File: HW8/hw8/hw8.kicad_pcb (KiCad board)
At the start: 2 copper layers, 27 parts, among them J1 Barrel_Jack, J2 Conn_01x02_Pin, J3 Comm 1 Terminal, J4 Conn_01x02_Pin, J5 Comm 2 Terminal, K1 SANYOU_SRD_Form_C, K2 SANYOU_SRD_Form_C, Q1 BC337, Q2 BC337, U1 LM317_TO-220, U2 PC817, U3 PC817

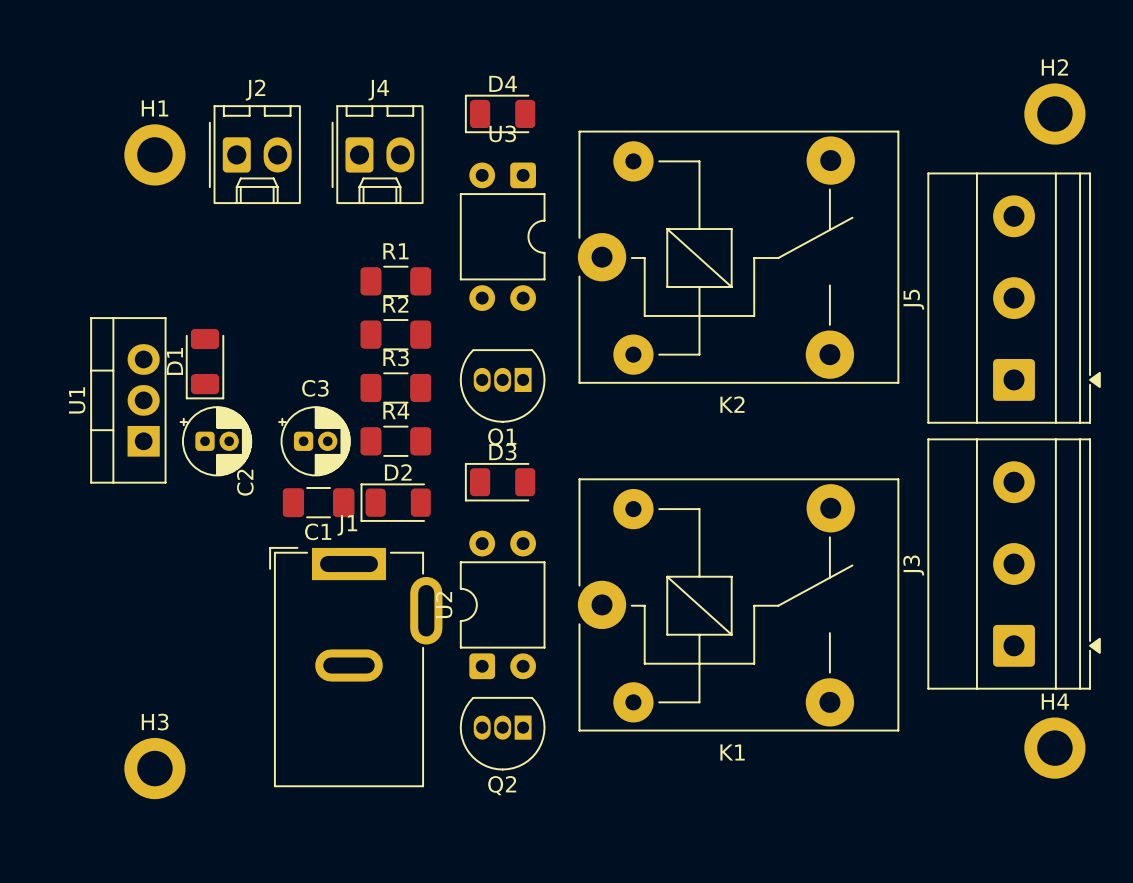
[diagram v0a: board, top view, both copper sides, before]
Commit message: hw9 done
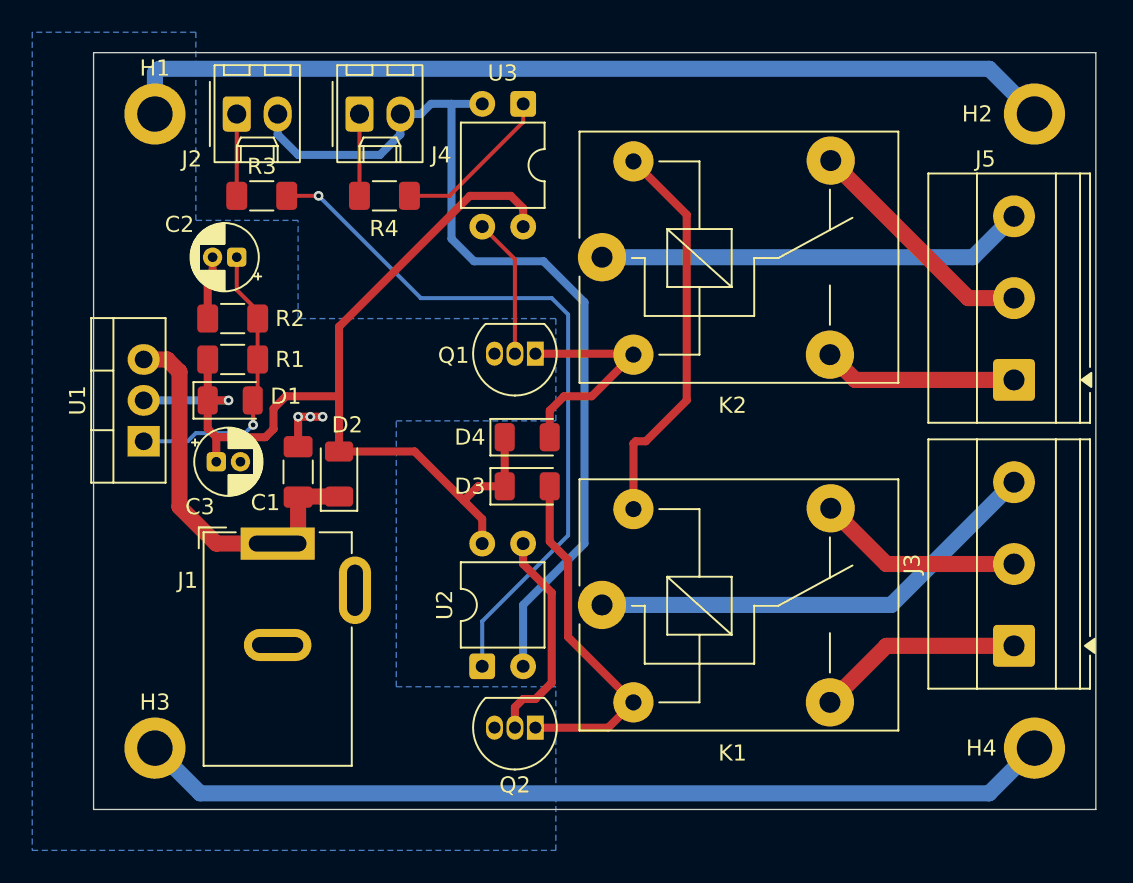
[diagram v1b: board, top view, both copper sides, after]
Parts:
- moved D4 20.1 mm to (119.6, 49.3)
- moved R4 15.3 mm to (110.8, 34.3)
- moved R3 14.6 mm to (103.2, 34.3)
- moved C2 11.6 mm to (101.6, 38.1), turned to 180 degrees
- moved R1 11.2 mm to (101.3, 44.5)
- moved R2 10.2 mm to (101.3, 41.9)
- moved C3 5.57 mm to (100.3, 50.8)
- moved J1 4.61 mm to (104.1, 55.9)
- moved U3 4.44 mm to (119.4, 28.6)
- moved D2 4.09 mm to (108.0, 51.6), turned to 90 degrees
- moved D1 2.87 mm to (101.2, 47.0), turned to 0 degrees
- moved H1 2.54 mm to (96.5, 29.2)
- moved J2 2.54 mm to (101.6, 29.2)
- moved J4 2.54 mm to (109.2, 29.2)
- moved C1 2.29 mm to (105.4, 51.4), turned to 90 degrees
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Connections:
- K1 pad 3: Net-(J3-Pin_2) -> Net-(J3-Pin_1)
- K1 pad 4: Net-(J3-Pin_1) -> Net-(J3-Pin_2)
- K2 pad 3: Net-(J5-Pin_2) -> Net-(J5-Pin_1)
- K2 pad 4: Net-(J5-Pin_1) -> Net-(J5-Pin_2)
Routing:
- net GND: track 0.00 -> 122.1 mm, vias 0 -> 3
- net +5V: track 0.00 -> 89.4 mm, vias 0 -> 1
- net GNDS: track 0.00 -> 59.0 mm
- net Net-(R3-Pad2): track 0.00 -> 44.6 mm, vias 0 -> 1
- net Net-(J3-Pin_3): track 0.00 -> 28.7 mm
- net Net-(J5-Pin_3): track 0.00 -> 26.6 mm
- net +12V: track 0.00 -> 23.4 mm
- net Net-(D3-A): track 0.00 -> 22.3 mm
- net Net-(D1-A): track 0.00 -> 18.3 mm, vias 0 -> 1
- net Net-(J5-Pin_2): track 0.00 -> 14.9 mm
- net Net-(D4-A): track 0.00 -> 14.4 mm
- net Net-(Q2-B): track 0.00 -> 13.6 mm
- net Net-(J3-Pin_1): track 0.00 -> 12.9 mm
- net Net-(J3-Pin_2): track 0.00 -> 12.8 mm
- net Net-(J5-Pin_1): track 0.00 -> 12.1 mm
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- added copper zone on B.Cu, net GND
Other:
- board outline added: 62.2 x 47 mm
